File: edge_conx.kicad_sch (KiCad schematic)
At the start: 14 parts, among them J113 Conn_02x12_Pin, J114 Conn_02x02_Pin, J115 Conn_02x10_Pin, J116 Conn_02x06_Pin, J117 Conn_02x12_Pin, J118 Conn_02x02_Pin, J119 Conn_02x10_Pin, J120 Conn_02x06_Pin, J121 Conn_02x06_Pin, J122 Conn_02x06_Pin, J123 Conn_02x06_Pin, J124 Conn_02x06_Pin, J125 Conn_02x06_Pin, J126 Conn_02x06_Pin

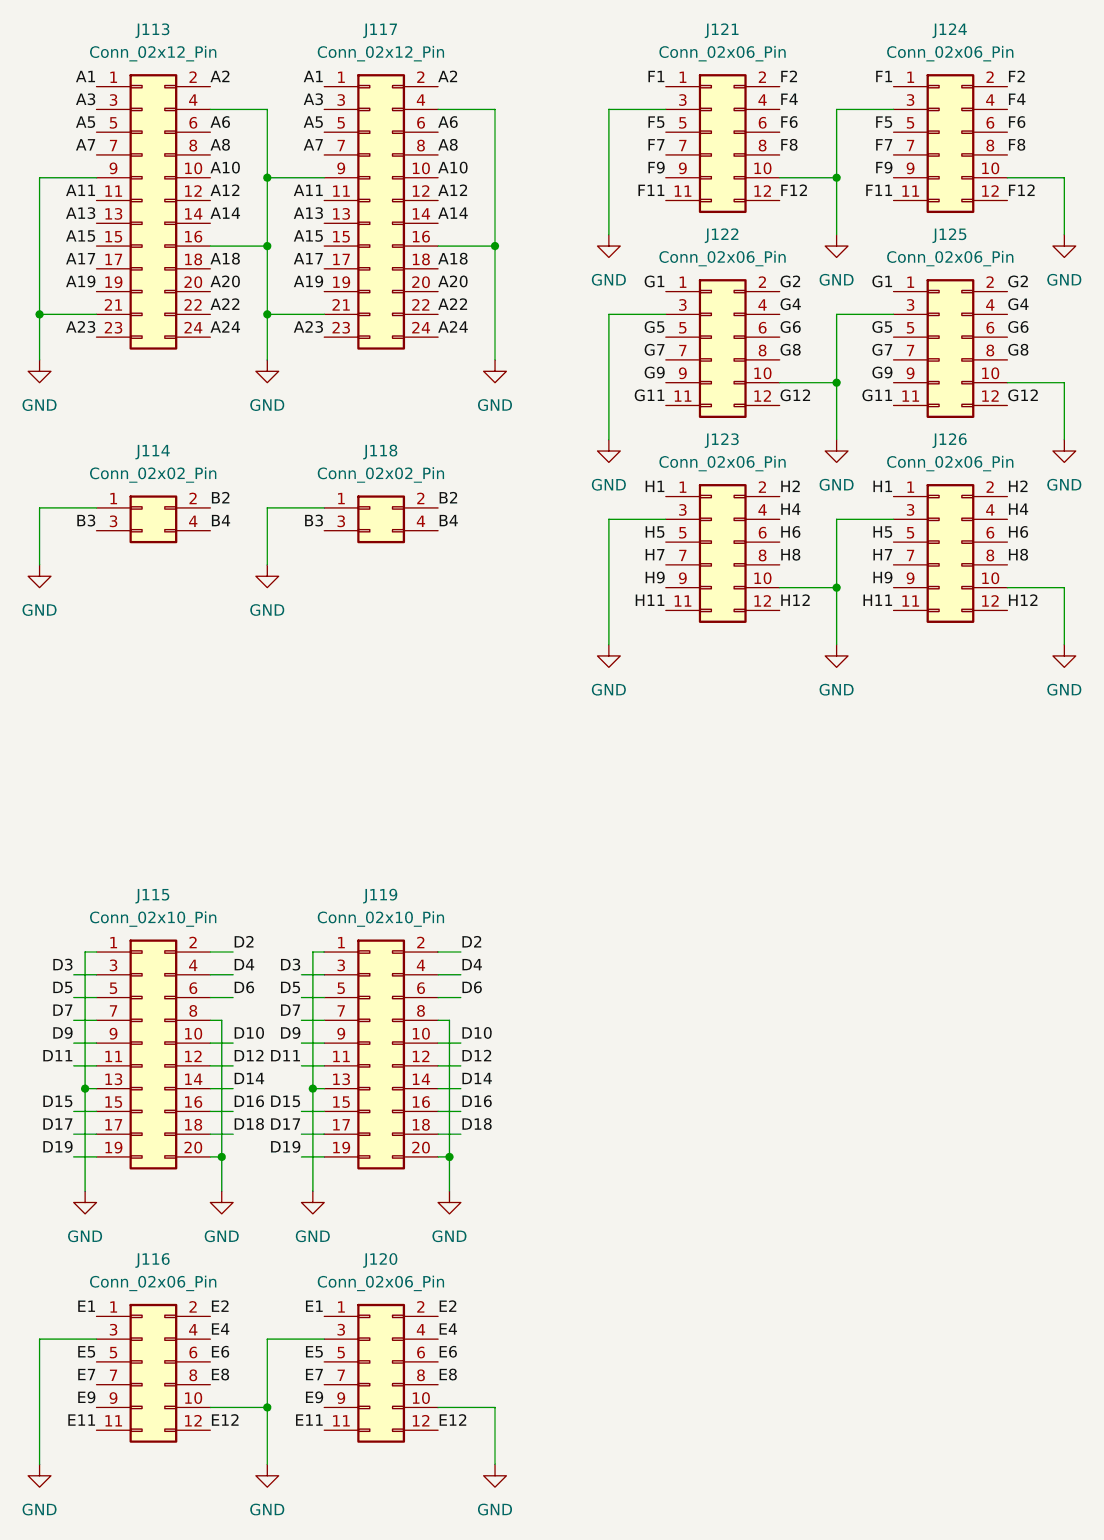
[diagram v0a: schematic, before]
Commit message: Edge connector changes
Probably a number of other unassorted changes as well.
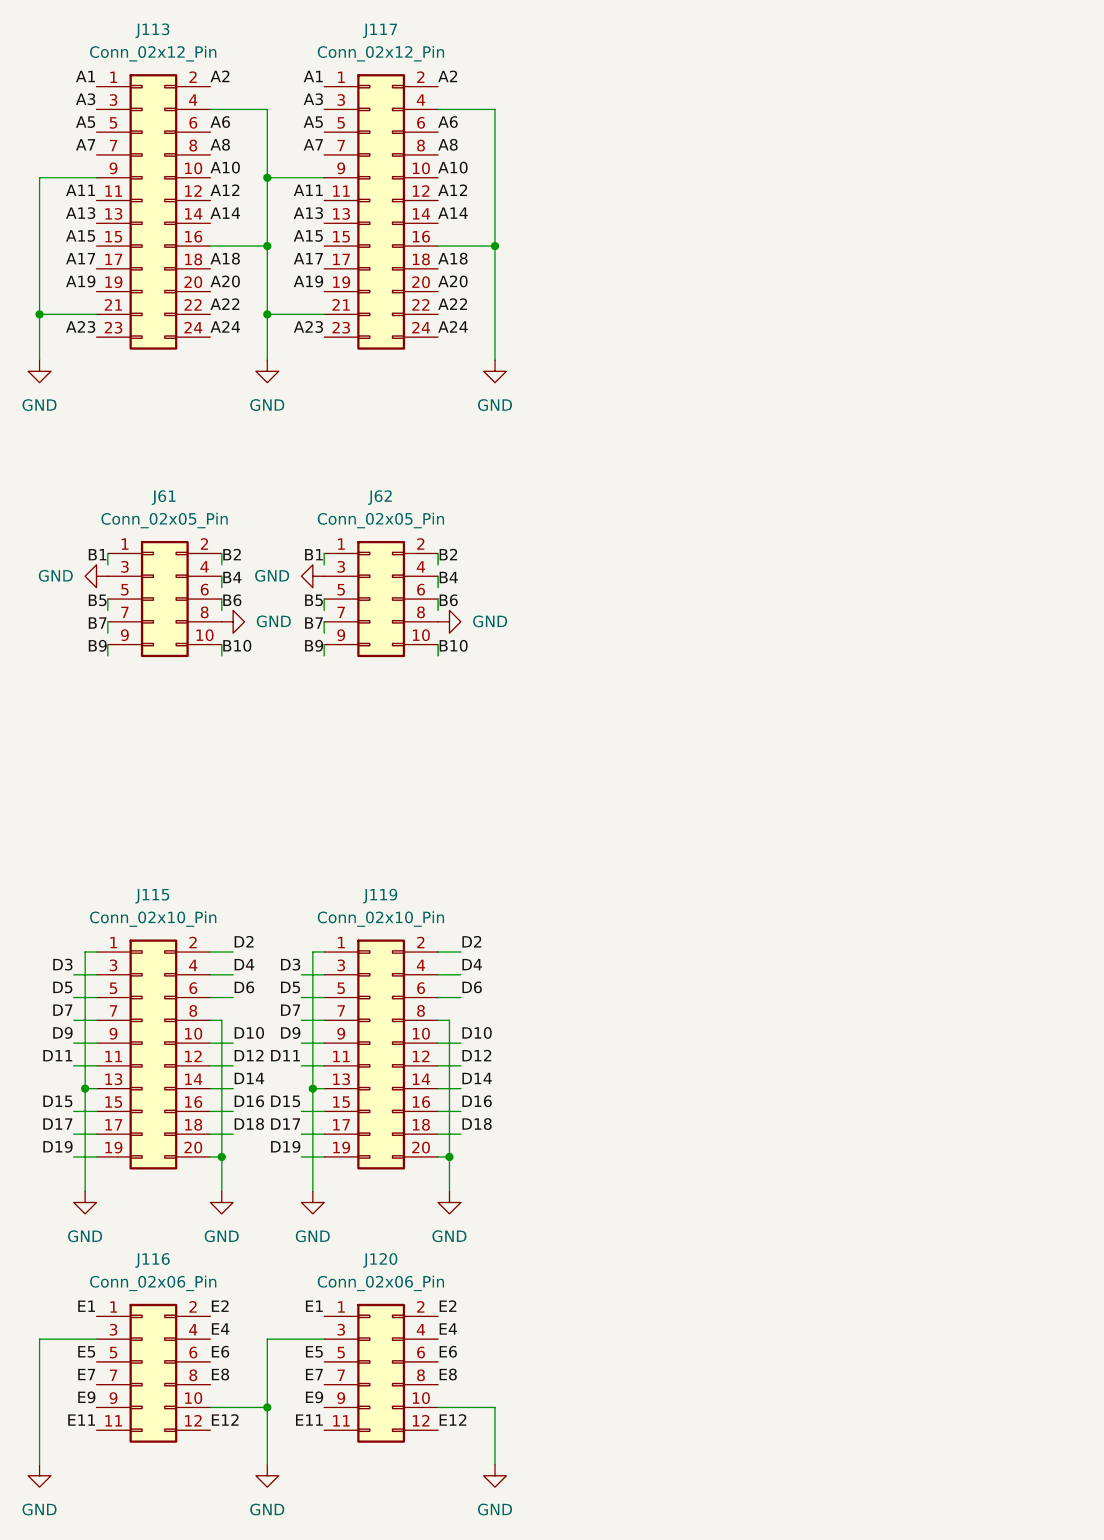
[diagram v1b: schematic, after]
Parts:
- removed J114: Conn_02x02_Pin, HL_Connector_Pad_2.54mm:Pad_2x02_P2.54_1.7x1.7_1Rect-3Oct, symbol Connector_Generic:Conn_02x02_Odd_Even
- removed J118: Conn_02x02_Pin, HL_Connector_Pad_2.54mm:Pad_2x02_P2.54_1.7x1.7_1Rect-3Oct_Mirror, symbol Connector_Generic:Conn_02x02_Odd_Even
- removed J121, J122, J123, J124, J125, J126: Conn_02x06_Pin, HL_Connector_Pad_2.54mm:Pad_2x06_P2.54_1.7x1.7_2Rect-10Oct, symbol Connector_Generic:Conn_02x06_Odd_Even
- added J61, J62: Conn_02x05_Pin, HL_Connector_Pad_2.54mm:Pad_2x05_P2.54_1.7x1.7_2Rect-8Oct, symbol Connector_Generic:Conn_02x05_Odd_Even
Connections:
- net B2: now also J61.2 (Pin_2), J62.2 (Pin_2)
- net B4: now also J61.4 (Pin_4), J62.4 (Pin_4)
- net GND: now also J61.3 (Pin_3), J61.8 (Pin_8), J62.3 (Pin_3), J62.8 (Pin_8)
- new net B1: J61.1 (Pin_1), J62.1 (Pin_1)
- new net B10: J61.10 (Pin_10), J62.10 (Pin_10)
- new net B5: J61.5 (Pin_5), J62.5 (Pin_5)
- new net B6: J61.6 (Pin_6), J62.6 (Pin_6)
- new net B7: J61.7 (Pin_7), J62.7 (Pin_7)
- new net B9: J61.9 (Pin_9), J62.9 (Pin_9)
